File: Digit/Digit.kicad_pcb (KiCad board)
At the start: 2 copper layers, 43.4 x 93 mm, 43 parts, among them J1 4s Batt, J10 Linear Actuator, J2 12V, J3 VIC CAN, J4 Debug, J5 EF Motor, J6 Cam 1 Pwr Conn, J7 Lynx Servos, J8 EF Laser, J9 CAM 12V, Q2 SSM3K329R_LF, U1 TJA1051T/3, U2 BD6220F

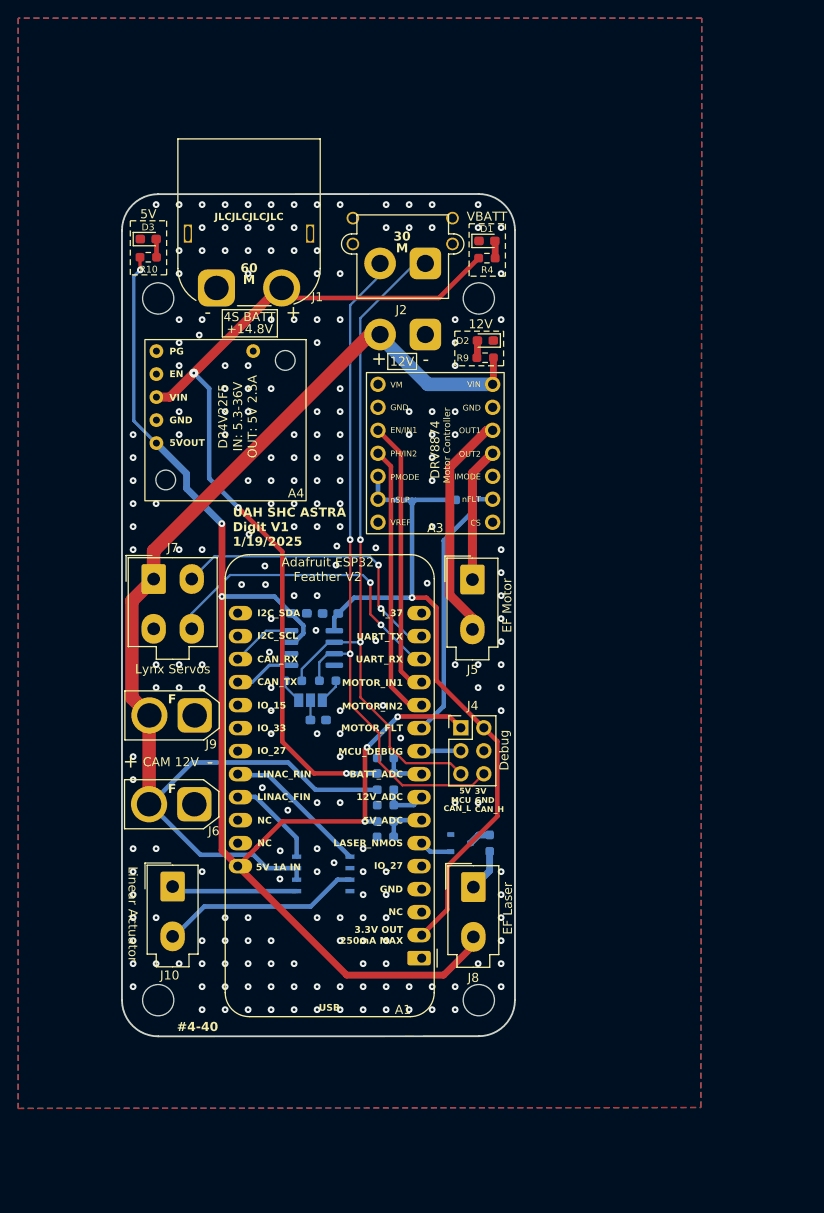
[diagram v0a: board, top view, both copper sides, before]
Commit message: URC '25 - V2
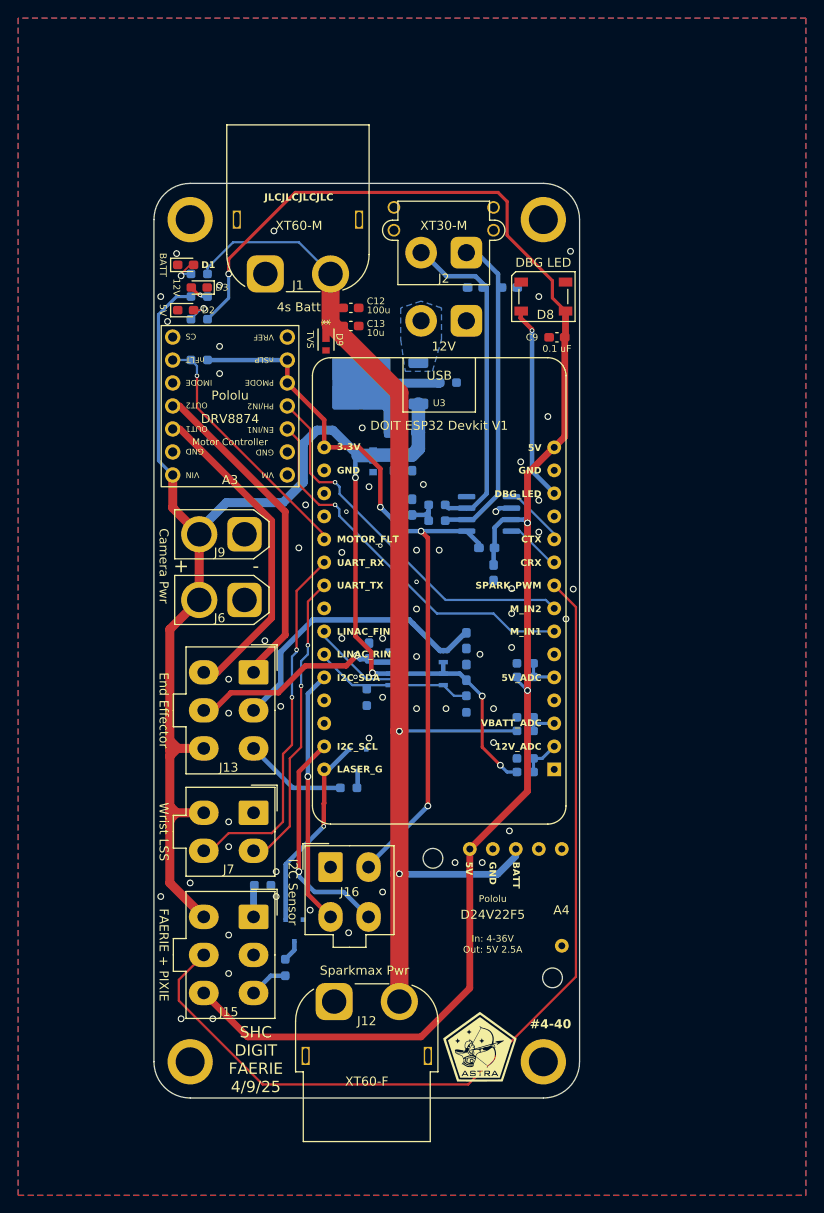
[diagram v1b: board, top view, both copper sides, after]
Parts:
- removed A1: Adafruit Feather ESP32 V2, Module:Adafruit_Feather
- removed the G*** at (46.2, 120.9)
- removed the G*** at (40.5, 58.2)
- removed the G*** at (59.1, 59.0)
- removed J10: Linear Actuator, Connector_Molex:Molex_Mini-Fit_Jr_5566-02A_2x01_P4.20mm_Vertical
- removed J4: Debug, Connector_PinHeader_2.54mm:PinHeader_2x03_P2.54mm_Vertical
- removed J5: EF Motor, Connector_Molex:Molex_Mini-Fit_Jr_5566-02A_2x01_P4.20mm_Vertical
- removed J8: EF Laser, Connector_Molex:Molex_Mini-Fit_Jr_5566-02A_2x01_P4.20mm_Vertical
- removed JP1: CAN Term Jmp, Jumper:SolderJumper-3_P1.3mm_Open_Pad1.0x1.5mm
- removed REF** (x3): 4-40 Mounting Hole, Digit:4-40 Mounting Hole
- removed REF**: 4-40, Digit:4-40 Mounting Hole
- added C10: 1uF, Capacitor_SMD:C_0603_1608Metric_Pad1.08x0.95mm_HandSolder, B.Cu at (62.5, 83.8)
- added C11: 1uF, Capacitor_SMD:C_0603_1608Metric_Pad1.08x0.95mm_HandSolder, B.Cu at (51.8, 84.9)
- added C12: 100u, Capacitor_SMD:C_0603_1608Metric_Pad1.08x0.95mm_HandSolder, F.Cu at (49.8, 47.0)
- added C13: 10u, Capacitor_SMD:C_0603_1608Metric_Pad1.08x0.95mm_HandSolder, F.Cu at (49.8, 49.0)
- added C2: 100u, Capacitor_SMD:C_0603_1608Metric_Pad1.08x0.95mm_HandSolder, B.Cu at (54.5, 64.1)
- added C5: 10u, Capacitor_SMD:C_0603_1608Metric_Pad1.08x0.95mm_HandSolder, B.Cu at (56.5, 64.1)
- added C6: 100pF, Capacitor_SMD:C_0603_1608Metric_Pad1.08x0.95mm_HandSolder, B.Cu at (67.2, 44.8)
- added C7: 100pF, Capacitor_SMD:C_0603_1608Metric_Pad1.08x0.95mm_HandSolder, B.Cu at (63.5, 44.8)
- added C8: 10uF, Capacitor_SMD:C_0603_1608Metric_Pad1.08x0.95mm_HandSolder, B.Cu at (62.5, 87.2)
- added C9: 0.1 uF, Capacitor_SMD:C_0603_1608Metric_Pad1.08x0.95mm_HandSolder, F.Cu at (72.5, 50.2)
- added D4: TVS, SHC:SOD-323HEUS2H_TOS, B.Cu at (52.2, 63.9)
- added D5: 15, Diode_SMD:D_SOD-123, B.Cu at (55.5, 60.8)
- added D8: Inolux_IN-PI554FCH, LED_SMD:LED_Inolux_IN-PI554FCH_PLCC4_5.0x5.0mm_P3.2mm, F.Cu at (71.0, 45.8)
- added D9: TVS, SHC:SOD-323HEUS2H_TOS, F.Cu at (47.0, 50.5)
- added G***: LOGO, LOGO, F.Cu at (64.0, 128.5)
- added G***: LOGO, LOGO, B.Cu at (68.5, 56.0)
- added G***: LOGO, LOGO, B.Cu at (63.5, 118.0)
- added H1: MountingHole_3.2mm_M3, MountingHole:MountingHole_3.2mm_M3, F.Cu at (32.0, 37.2)
- added H2: MountingHole_3.2mm_M3, MountingHole:MountingHole_3.2mm_M3, F.Cu at (71.0, 37.2)
- added H3: MountingHole_3.2mm_M3, MountingHole:MountingHole_3.2mm_M3, F.Cu at (32.0, 130.2)
- added H4: MountingHole_3.2mm_M3, MountingHole:MountingHole_3.2mm_M3, F.Cu at (71.0, 130.2)
- added J12: Sparkmax Pwr, Connector_AMASS:AMASS_XT60PW-F_1x02_P7.20mm_Horizontal, F.Cu at (47.9, 123.6)
- added J13: EF Motor, Lin ac, Laser, Connector_Molex:Molex_Mini-Fit_Jr_5566-06A_2x03_P4.20mm_Vertical, F.Cu at (39.0, 87.2)
- added J15: UV Bulb, Sparkmax PWM, Lasers, Connector_Molex:Molex_Mini-Fit_Jr_5566-06A_2x03_P4.20mm_Vertical, F.Cu at (39.0, 114.2)
- added J16: AS7341 or SHT30, Connector_Molex:Molex_Mini-Fit_Jr_5566-04A_2x02_P4.20mm_Vertical, F.Cu at (47.5, 108.8)
- added Q3: PMOS, Package_TO_SOT_SMD:TO-252-2, B.Cu at (52.2, 55.3)
- added Q4: SSM3K329R_LF, Digit:SOT-23F_TOS, B.Cu at (50.5, 96.9)
- added R14: 10k, Resistor_SMD:R_0603_1608Metric_Pad0.98x0.95mm_HandSolder, B.Cu at (51.5, 90.0)
- added R16: 10, Resistor_SMD:R_0603_1608Metric_Pad0.98x0.95mm_HandSolder, B.Cu at (49.5, 100.0)
- added R17: 50k, Resistor_SMD:R_0603_1608Metric_Pad0.98x0.95mm_HandSolder, B.Cu at (60.5, 55.2)
- added R18: 330, Resistor_SMD:R_0603_1608Metric_Pad0.98x0.95mm_HandSolder, B.Cu at (40.0, 110.8)
- added R19: 0Ω, Resistor_SMD:R_0603_1608Metric_Pad0.98x0.95mm_HandSolder, B.Cu at (42.5, 119.8)
- added U3: ESP32 DOIT Devkit V1, esp32_devkit_v1_doit:esp32_devkit_v1_doit, F.Cu at (59.5, 98.0)
- C3: value 0.1 μF -> 100 nF
- C4: value 1.0 μF -> 47 nF
- D1: value VBATT -> BATT
- J9: value CAM 12V -> CAM 2 Pwr Conn
- Q2: footprint Libraries:SOTFL95P240X88-3N -> Digit:SOT-23F_TOS
- R1: value 10Ω -> 10k
- R10, R4, R9: moved to B.Cu
- R11, R12: value 60Ω -> 60
- R2, R3, R5, R7: value 10 kΩ -> 10k
- R6: value 3.8 kΩ -> 3.32k
- R8: value 3.1 kΩ -> 2.21k
- U2: value BD6220F -> BD622xF
- moved A4 78.5 mm to (74.3, 123.3), turned to 180 degrees
- moved D1 33.4 mm to (31.5, 42.2)
- moved R13 33.1 mm to (33.0, 52.8), turned to 180 degrees
- moved R9 32.3 mm to (33.0, 45.8), turned to 0 degrees
- moved D2 32.1 mm to (33.0, 44.8)
- moved R4 31.8 mm to (33.0, 43.2), turned to 180 degrees
- moved J7 28.1 mm to (39.0, 102.8), turned to -90 degrees
- moved C1 25.7 mm to (56.5, 69.0), turned to -90 degrees
- moved U2 25.0 mm to (57.0, 86.8), turned to 180 degrees
- moved R3 24.6 mm to (69.0, 86.2)
- moved U1 24.5 mm to (65.0, 69.8), turned to 180 degrees
- moved A3 24.2 mm to (44.0, 49.0), turned to 180 degrees
- moved R12 23.7 mm to (59.2, 70.5)
- moved J6 23.2 mm to (38.0, 79.2)
- moved R11 22.9 mm to (59.2, 68.8), turned to 180 degrees
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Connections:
- C1 pad 2: Net-(JP1-C) -> Net-(C1-Pad2)
- C3 pad 1: GND -> +5V
- J2 pad 2: +12V -> /12V_IN
- J7 pad 1: +12V -> GND
- J7 pad 3: GND -> +12V
- R1 pad 1: Net-(Q2-Pad3) -> GND
- R1 pad 2: Net-(J8-Pin_1) -> /LINAC_FIN
- R11 pad 2: Net-(JP1-A) -> Net-(C1-Pad2)
- R12 pad 1: Net-(JP1-B) -> Net-(C1-Pad2)
- U2 pad 6: unconnected-(U2-VREF-Pad6) -> +12V
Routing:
- net /SPARK_PWM: track 0.00 -> 103.0 mm
- net +12V: track 131.2 -> 178.3 mm, vias 0 -> 4
- net /CAN_L: track 76.5 -> 35.9 mm, vias 2 -> 0
- net /CAN_H: track 76.5 -> 37.0 mm, vias 2 -> 0
- net +BATT: track 99.6 -> 127.9 mm, vias 3 -> 2
- net /I2C_SDA: track 0.00 -> 28.2 mm, vias 0 -> 1
- net /I2C_SCL: track 0.00 -> 25.1 mm, vias 0 -> 1
- net +5V: track 156.8 -> 179.7 mm, vias 6 -> 3
- net /NEO_LED_DIN: track 0.00 -> 21.7 mm, vias 0 -> 1
- net /MOTOR_OUT2: track 14.9 -> 36.5 mm
- net /LASER_NMOS: track 3.61 -> 22.0 mm, vias 0 -> 1
- net /LINAC_NEG: track 13.9 -> 31.9 mm
- net Net-(D5-A): track 0.00 -> 13.1 mm
- net /MOTOR_IN1: track 30.4 -> 42.0 mm, vias 0 -> 1
- net /MOTOR_IN2: track 30.6 -> 42.1 mm, vias 0 -> 1
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- added copper zone on B.Cu, net /12V_IN
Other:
- board size 43.4 x 93 mm -> 47 x 101 mm
- rule pad_to_mask_clearance: 0 -> 0.038
- board text added: "3.3V"
- board text added: "3V3"
- board text added: "4s Batt"
- board text added: "BD6620F"
- board text added: "CRX"
- board text added: "CTX"
- board text added: "Camera Pwr"
- board text added: "D24V22F5 5V Buck"
- board text added: "DBG LED"
- board text added: "DBG_LED"
- board text added: "DOIT ESP32 Devkit V1"
- board text added: "EF Motor"
- board text added: "End Effector"
- board text added: "FAERIE + DIGIT ASTRA, SHC at UAH 47 x 101 mm"
- board text added: "FAERIE + PIXIE"
- board text added: "H"
- board text added: "I2C Sensor"
- board text added: "I2C Sensors"
- board text added: "In: 4-36V Out: 5V 2.5A"
- board text added: "L"
- board text added: "LASER_G"
- board text added: "Laser"
- board text added: "Lin Ac"
- board text added: "Lynxmotion Servos"
- board text added: "M_IN1"
- board text added: "M_IN2"
- board text added: "NEG"
- board text added: "NMOS"
- board text added: "PJD60P04E-AU"
- board text added: "POS"
- board text added: "PWM"
- board text added: "Pololu"
- board text added: "Pololu DRV8874 Motor Controller"
- board text added: "SCL"
- board text added: "SDA"
- board text added: "SHC DIGIT FAERIE 4/9/25"
- board text added: "SPARK_PWM"
- board text added: "Spark"
- board text added: "SparkMax Pwr"
- board text added: "Sparkmax Pwr"
- board text added: "TJA1051T/3"
- board text added: "TVS"
- board text added: "UV LED"
- board text added: "VBATT"
- board text added: "VBATT_ADC"
- board text added: "Vic CAN"
- board text added: "Wrist LSS"
- board text added: "XT30-M"
- board text added: "XT60-F"
- board text added: "XT60-M"
- board text added: "Zener"
- board text removed: "+"
- board text removed: "+14.8V"
- board text removed: "-"
- board text removed: "3.3V OUT 250mA MAX"
- board text removed: "30"
- board text removed: "3V"
- board text removed: "4S BATT"
- board text removed: "5V 1A IN"
- board text removed: "5VOUT"
- board text removed: "60"
- board text removed: "Adafruit ESP32 Feather V2"
- board text removed: "BATT_ADC"
- board text removed: "CAN Transceiver"
- board text removed: "CAN_H"
- board text removed: "CAN_L"
- board text removed: "CAN_RX"
- board text removed: "CAN_TX"
- board text removed: "D"
- board text removed: "David Sharpe Digit V1 43.4 x 93.0 mm"
- board text removed: "EN"
- board text removed: "F"
- board text removed: "G"
- board text removed: "IN: 5.3-36V OUT: 5V 2.5A"
- board text removed: "IO_15"
- board text removed: "IO_27"
- board text removed: "IO_33"
- board text removed: "I_37"
- board text removed: "LASER_NMOS"
- board text removed: "M"
- board text removed: "MCU"
- board text removed: "MCU_DEBUG"
- board text removed: "MOTOR_IN1"
- board text removed: "MOTOR_IN2"
- board text removed: "NC"
- board text removed: "PG"
- board text removed: "S"
- board text removed: "UAH SHC ASTRA Digit V1 1/19/2025"
- board text removed: "USB"
- board text removed: "VIN"
